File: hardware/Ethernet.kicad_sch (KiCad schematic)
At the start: 28 parts, among them IC1 DP83826AIRHBR, J5 RJ45_Pulse_JXD6-0001NL, J8 Conn_01x04, Y1 SiT8008AI-32-33E-50.000000

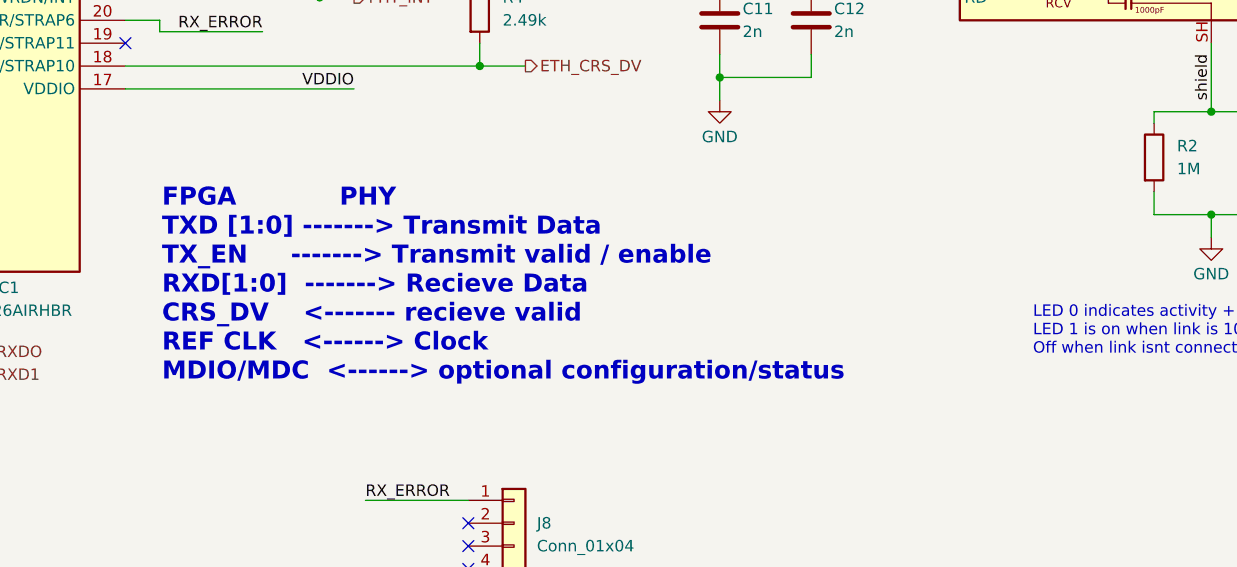
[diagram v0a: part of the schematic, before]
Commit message: most of layout is done, only have single ended highspeed signals left. mika pleaaaaaaaaaaaaaaaaaseeeeeeee review :beg:
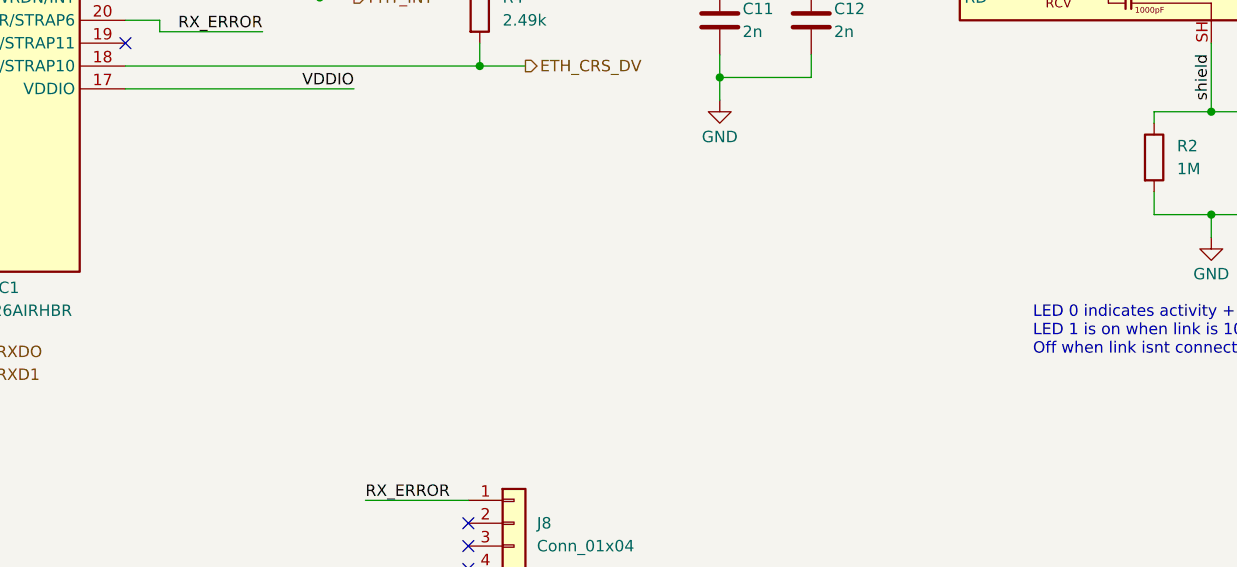
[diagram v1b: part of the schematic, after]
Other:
- note removed: "FPGA PHY TXD [1:0] -------> Transmit Data TX_EN -------> Transmit valid / enable RXD[1:0] -------> Recieve Data CRS_DV <------- recieve valid REF CLK <------> Clock MDIO/MDC <------> optional configuration/status"
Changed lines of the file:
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@@
-		)
-	)
-	(text "FPGA			PHY\nTXD [1:0] -------> Transmit Data\nTX_EN     -------> Transmit valid / enable\nRXD[1:0]  -------> Recieve Data\nCRS_DV    <------- recieve valid\nREF CLK   <------> Clock\nMDIO/MDC  <------> optional configuration/status"
-		(exclude_from_sim no)
-		(at 143.764 122.174 0)
-		(effects
-			(font
-				(size 2 2)
-				(thickness 0.4)
-				(bold yes)
-			)
-			(justify left)
 		)
 	)
